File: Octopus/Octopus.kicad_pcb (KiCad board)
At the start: 2 copper layers, 160 x 100 mm, 54 parts, among them J1 MIDI IN (to panel DIN), J10 RN111PC, J2 9-12VDC IN, J3 RN111PC, J4 RN111PC, J5 RN111PC, J6 RN111PC, J7 RN111PC, J8 RN111PC, J9 RN111PC, K1 G5V-1, K2 G5V-1, K3 G5V-1, K4 G5V-1, K5 G5V-1, K6 G5V-1, K7 G5V-1, K8 G5V-1, U1 Teensy4.1, U2 6N138, U3 ULN2803A, U4 L7805

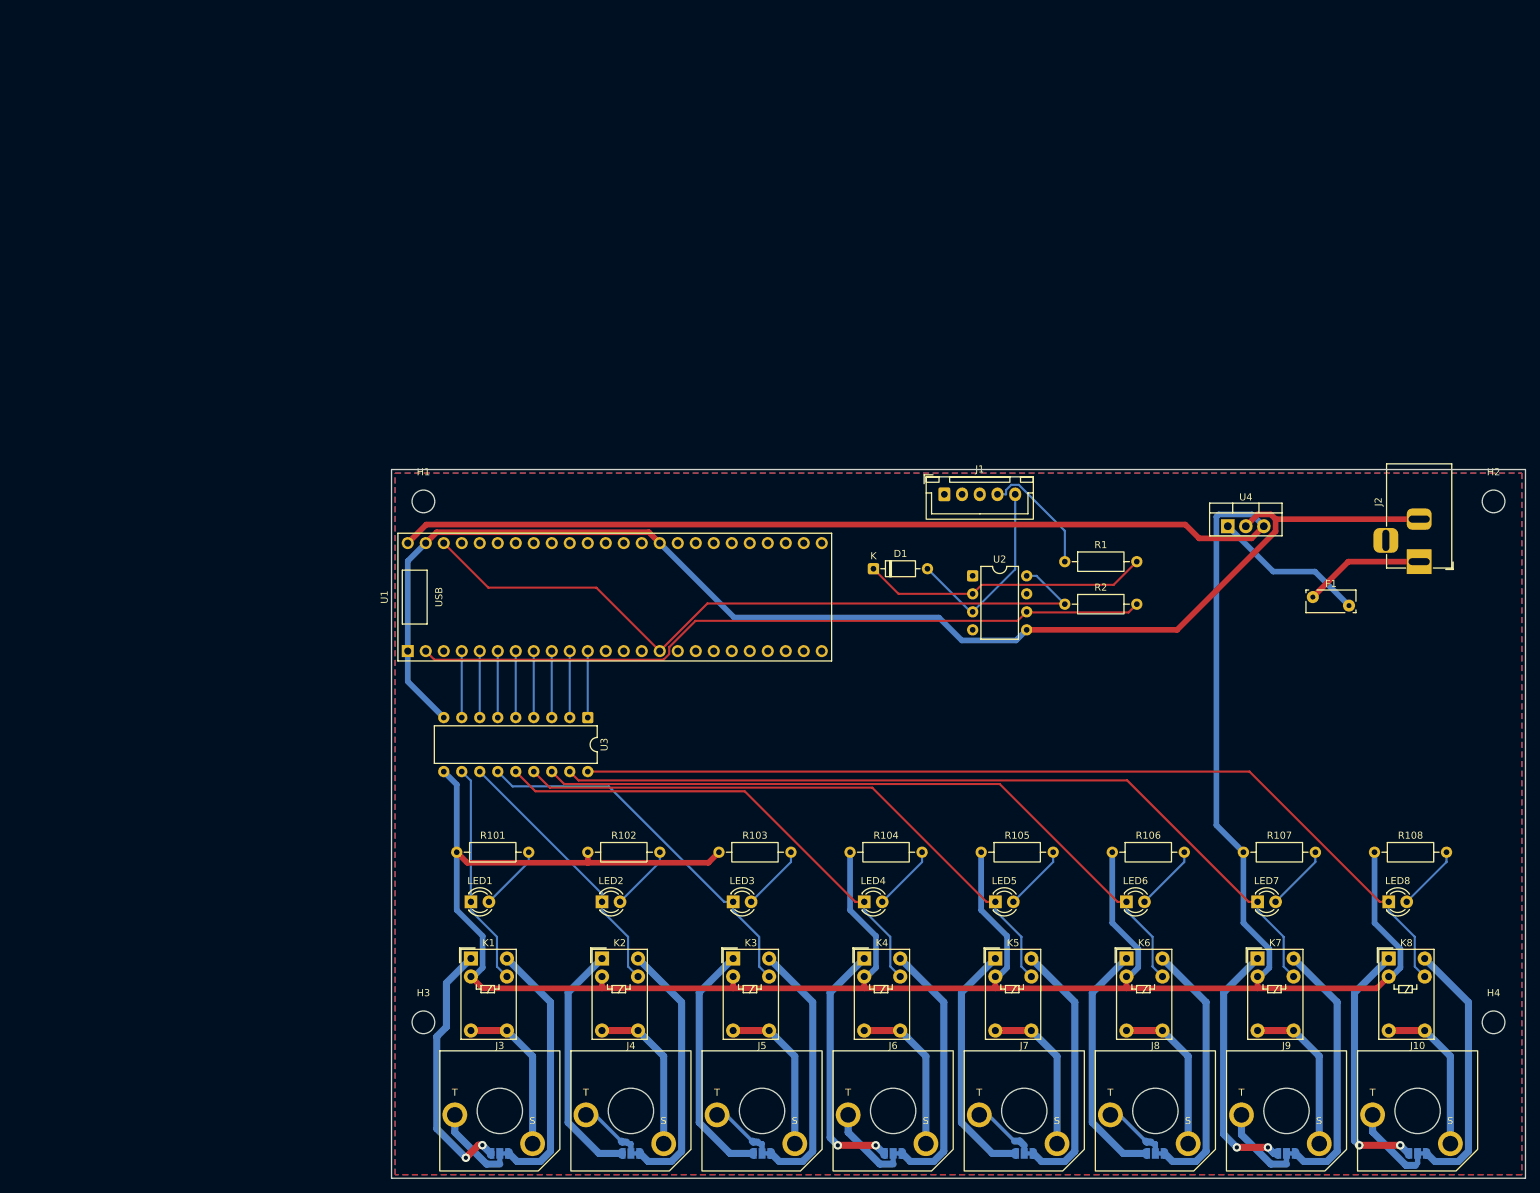
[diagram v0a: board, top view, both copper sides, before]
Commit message: Octopus updates
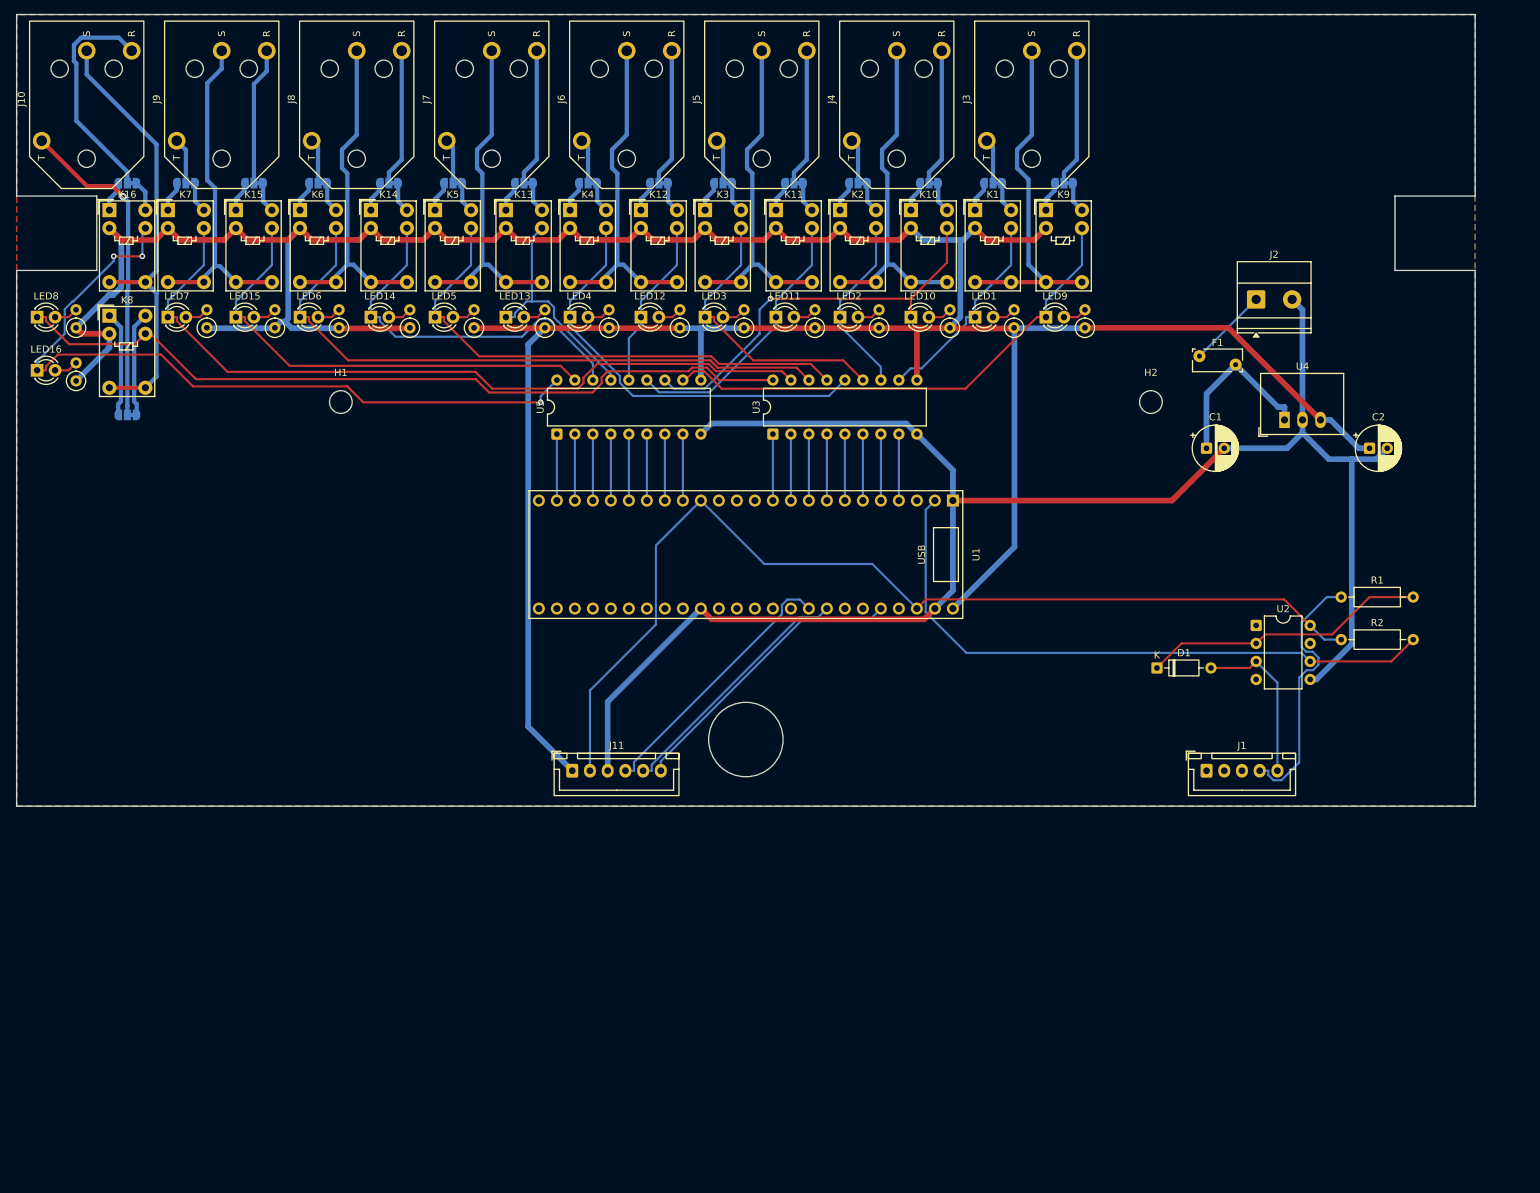
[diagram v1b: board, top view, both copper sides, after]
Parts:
- removed H3, H4: M3, MountingHole:MountingHole_3.2mm_M3
- added C1: 10uF 25V, Capacitor_THT:CP_Radial_D6.3mm_P2.50mm, F.Cu at (215.0, 97.0)
- added C2: 22uF 10V, Capacitor_THT:CP_Radial_D6.3mm_P2.50mm, F.Cu at (238.0, 97.0)
- added J11: Button panel, Connector_JST:JST_XH_B6B-XH-A_1x06_P2.50mm_Vertical, F.Cu at (125.5, 142.5)
- added JP10: NO|NC, Jumper:SolderJumper-3_P1.3mm_Bridged12_RoundedPad1.0x1.5mm, B.Cu at (175.8, 59.6)
- added JP11: NO|NC, Jumper:SolderJumper-3_P1.3mm_Bridged12_RoundedPad1.0x1.5mm, B.Cu at (156.8, 59.6)
- added JP12: NO|NC, Jumper:SolderJumper-3_P1.3mm_Bridged12_RoundedPad1.0x1.5mm, B.Cu at (137.7, 59.6)
- added JP13: NO|NC, Jumper:SolderJumper-3_P1.3mm_Bridged12_RoundedPad1.0x1.5mm, B.Cu at (118.7, 59.6)
- added JP14: NO|NC, Jumper:SolderJumper-3_P1.3mm_Bridged12_RoundedPad1.0x1.5mm, B.Cu at (99.6, 59.6)
- added JP15: NO|NC, Jumper:SolderJumper-3_P1.3mm_Bridged12_RoundedPad1.0x1.5mm, B.Cu at (80.6, 59.6)
- added JP16: NO|NC, Jumper:SolderJumper-3_P1.3mm_Bridged12_RoundedPad1.0x1.5mm, B.Cu at (62.7, 59.6)
- added JP9: NO|NC, Jumper:SolderJumper-3_P1.3mm_Bridged12_RoundedPad1.0x1.5mm, B.Cu at (194.9, 59.6)
- added K10: G5V-1, Relay_THT:Relay_SPDT_Omron_G5V-1, F.Cu at (173.3, 63.4)
- added K11: G5V-1, Relay_THT:Relay_SPDT_Omron_G5V-1, F.Cu at (154.2, 63.4)
- added K12: G5V-1, Relay_THT:Relay_SPDT_Omron_G5V-1, F.Cu at (135.2, 63.4)
- added K13: G5V-1, Relay_THT:Relay_SPDT_Omron_G5V-1, F.Cu at (116.1, 63.4)
- added K14: G5V-1, Relay_THT:Relay_SPDT_Omron_G5V-1, F.Cu at (97.1, 63.4)
- added K15: G5V-1, Relay_THT:Relay_SPDT_Omron_G5V-1, F.Cu at (78.0, 63.4)
- added K16: G5V-1, Relay_THT:Relay_SPDT_Omron_G5V-1, F.Cu at (60.2, 63.4)
- added K9: G5V-1, Relay_THT:Relay_SPDT_Omron_G5V-1, F.Cu at (192.3, 63.4)
- added LED10: LED, LED_THT:LED_D3.0mm, F.Cu at (173.3, 78.5)
- added LED11: LED, LED_THT:LED_D3.0mm, F.Cu at (154.2, 78.5)
- added LED12: LED, LED_THT:LED_D3.0mm, F.Cu at (135.2, 78.5)
- added LED13: LED, LED_THT:LED_D3.0mm, F.Cu at (116.1, 78.5)
- added LED14: LED, LED_THT:LED_D3.0mm, F.Cu at (97.1, 78.5)
- added LED15: LED, LED_THT:LED_D3.0mm, F.Cu at (78.0, 78.5)
- added LED16: LED, LED_THT:LED_D3.0mm, F.Cu at (50.0, 86.0)
- added LED9: LED, LED_THT:LED_D3.0mm, F.Cu at (192.3, 78.5)
- added R109: 1k, Resistor_THT:R_Axial_DIN0207_L6.3mm_D2.5mm_P2.54mm_Vertical, F.Cu at (197.8, 80.0)
- added R110: 1k, Resistor_THT:R_Axial_DIN0207_L6.3mm_D2.5mm_P2.54mm_Vertical, F.Cu at (178.8, 80.0)
- added R111: 1k, Resistor_THT:R_Axial_DIN0207_L6.3mm_D2.5mm_P2.54mm_Vertical, F.Cu at (159.7, 80.0)
- added R112: 1k, Resistor_THT:R_Axial_DIN0207_L6.3mm_D2.5mm_P2.54mm_Vertical, F.Cu at (140.7, 80.0)
- added R113: 1k, Resistor_THT:R_Axial_DIN0207_L6.3mm_D2.5mm_P2.54mm_Vertical, F.Cu at (121.6, 80.0)
- added R114: 1k, Resistor_THT:R_Axial_DIN0207_L6.3mm_D2.5mm_P2.54mm_Vertical, F.Cu at (102.6, 80.0)
- added R115: 1k, Resistor_THT:R_Axial_DIN0207_L6.3mm_D2.5mm_P2.54mm_Vertical, F.Cu at (83.5, 80.0)
- added R116: 1k, Resistor_THT:R_Axial_DIN0207_L6.3mm_D2.5mm_P2.54mm_Vertical, F.Cu at (55.5, 87.5)
- added U5: ULN2803A, Package_DIP:DIP-18_W7.62mm, F.Cu at (123.3, 95.0)
- J10, J3, J4, J5, J6, J7, J8, J9: value RN111PC -> RN112BPC; footprint Octopus:Jack_6.35mm_Switchcraft_RN111PC_Vertical -> Octopus:Jack_6.35mm_Switchcraft_RN112BPC_Horizontal
- J2: footprint Connector_BarrelJack:BarrelJack_Horizontal -> TerminalBlock_Phoenix:TerminalBlock_Phoenix_MKDS-1,5-2-5.08_1x02_P5.08mm_Horizontal
- R101, R102, R103, R104, R105, R106, R107, R108: footprint Resistor_THT:R_Axial_DIN0207_L6.3mm_D2.5mm_P10.16mm_Horizontal -> Resistor_THT:R_Axial_DIN0207_L6.3mm_D2.5mm_P2.54mm_Vertical
- U4: value L7805 -> R-78E5.0-1.0; footprint Package_TO_SOT_THT:TO-220-3_Vertical -> Converter_DCDC:Converter_DCDC_RECOM_R-78E-0.5_THT
- moved J10 243.7 mm to (57.0, 35.2), turned to 90 degrees
- moved J9 216.1 mm to (76.0, 35.2), turned to 90 degrees
- moved JP8 209.8 mm to (62.7, 92.3)
- moved LED8 207.8 mm to (50.0, 78.5)
- moved JP7 207.0 mm to (71.0, 59.6)
- moved K8 202.0 mm to (60.2, 78.3)
- moved R108 197.6 mm to (55.5, 80.0), turned to 90 degrees
- moved J8 191.9 mm to (95.1, 35.2), turned to 90 degrees
- moved K7 186.5 mm to (68.4, 63.4)
- moved JP6 180.8 mm to (89.6, 59.6)
- moved LED7 174.5 mm to (68.4, 78.5)
- moved J7 172.5 mm to (114.1, 35.2), turned to 90 degrees
- moved J3 172.5 mm to (190.3, 35.2), turned to 90 degrees
- moved R107 163.9 mm to (73.9, 80.0), turned to 90 degrees
- moved J6 159.8 mm to (133.2, 35.2), turned to 90 degrees
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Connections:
- net /CH1_COM renamed /JACK1_SLV
- net /CH1_TIP renamed /CH1_OUT
- net /CH2_COM renamed /JACK2_SLV
- net /CH2_TIP renamed /CH2_OUT
- net /CH3_COM renamed /JACK3_SLV
- net /CH3_TIP renamed /CH3_OUT
- net /CH4_COM renamed /JACK4_SLV
- net /CH4_TIP renamed /CH4_OUT
- net /CH5_COM renamed /JACK5_SLV
- net /CH5_TIP renamed /CH5_OUT
- net /CH6_COM renamed /JACK6_SLV
- net /CH6_TIP renamed /CH6_OUT
- net /CH7_COM renamed /JACK7_SLV
- net /CH7_TIP renamed /CH7_OUT
- net /CH8_COM renamed /JACK8_SLV
- net /CH8_TIP renamed /CH8_OUT
- net Net-(LED1-K) renamed /DRV1
- net Net-(LED2-K) renamed /DRV2
- net Net-(LED3-K) renamed /DRV3
- net Net-(LED4-K) renamed /DRV4
- net Net-(LED5-K) renamed /DRV5
- net Net-(LED6-K) renamed /DRV6
- net Net-(LED7-K) renamed /DRV7
- net Net-(LED8-K) renamed /DRV8
- U1 pad 18: (no net) -> /I2C_SDA
- U1 pad 19: (no net) -> /I2C_SCL
- U1 pad 22: (no net) -> /PANEL_INT
- U1 pad 24: (no net) -> Net-(U1-IO24)
- U1 pad 25: (no net) -> Net-(U1-IO25)
- U1 pad 26: (no net) -> Net-(U1-IO26)
- U1 pad 27: (no net) -> Net-(U1-IO27)
- U1 pad 28: (no net) -> Net-(U1-IO28)
- U1 pad 29: (no net) -> Net-(U1-IO29)
- U1 pad 30: (no net) -> Net-(U1-IO30)
- U1 pad 31: (no net) -> Net-(U1-IO31)
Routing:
- net /DRV16: track 0.00 -> 108.0 mm, vias 0 -> 3
- net /DRV9: track 0.00 -> 71.6 mm
- net /DRV15: track 0.00 -> 66.5 mm
- net /DRV10: track 0.00 -> 57.2 mm, vias 0 -> 1
- net GND: track 188.2 -> 243.0 mm
- net /DRV14: track 0.00 -> 53.4 mm
- net /PANEL_INT: track 0.00 -> 41.3 mm
- net /JACK8_SLV: track 22.5 -> 63.8 mm
- net +3V3: track 103.8 -> 144.2 mm
- net /DRV11: track 0.00 -> 38.7 mm
- net /I2C_SDA: track 0.00 -> 37.9 mm
- net /I2C_SCL: track 0.00 -> 35.9 mm
- net /CH8_OUT: track 12.2 -> 45.9 mm, vias 0 -> 1
- net /DRV13: track 0.00 -> 32.9 mm
- net /CH1_NO: track 36.7 -> 4.31 mm
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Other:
- board size 160 x 100 mm -> 205.8 x 111.7 mm
- board text added: "BACK PANEL (inside face)"
- board text added: "keep free: future mains PSU"
